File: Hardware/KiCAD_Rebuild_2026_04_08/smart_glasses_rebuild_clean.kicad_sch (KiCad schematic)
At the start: 12 parts

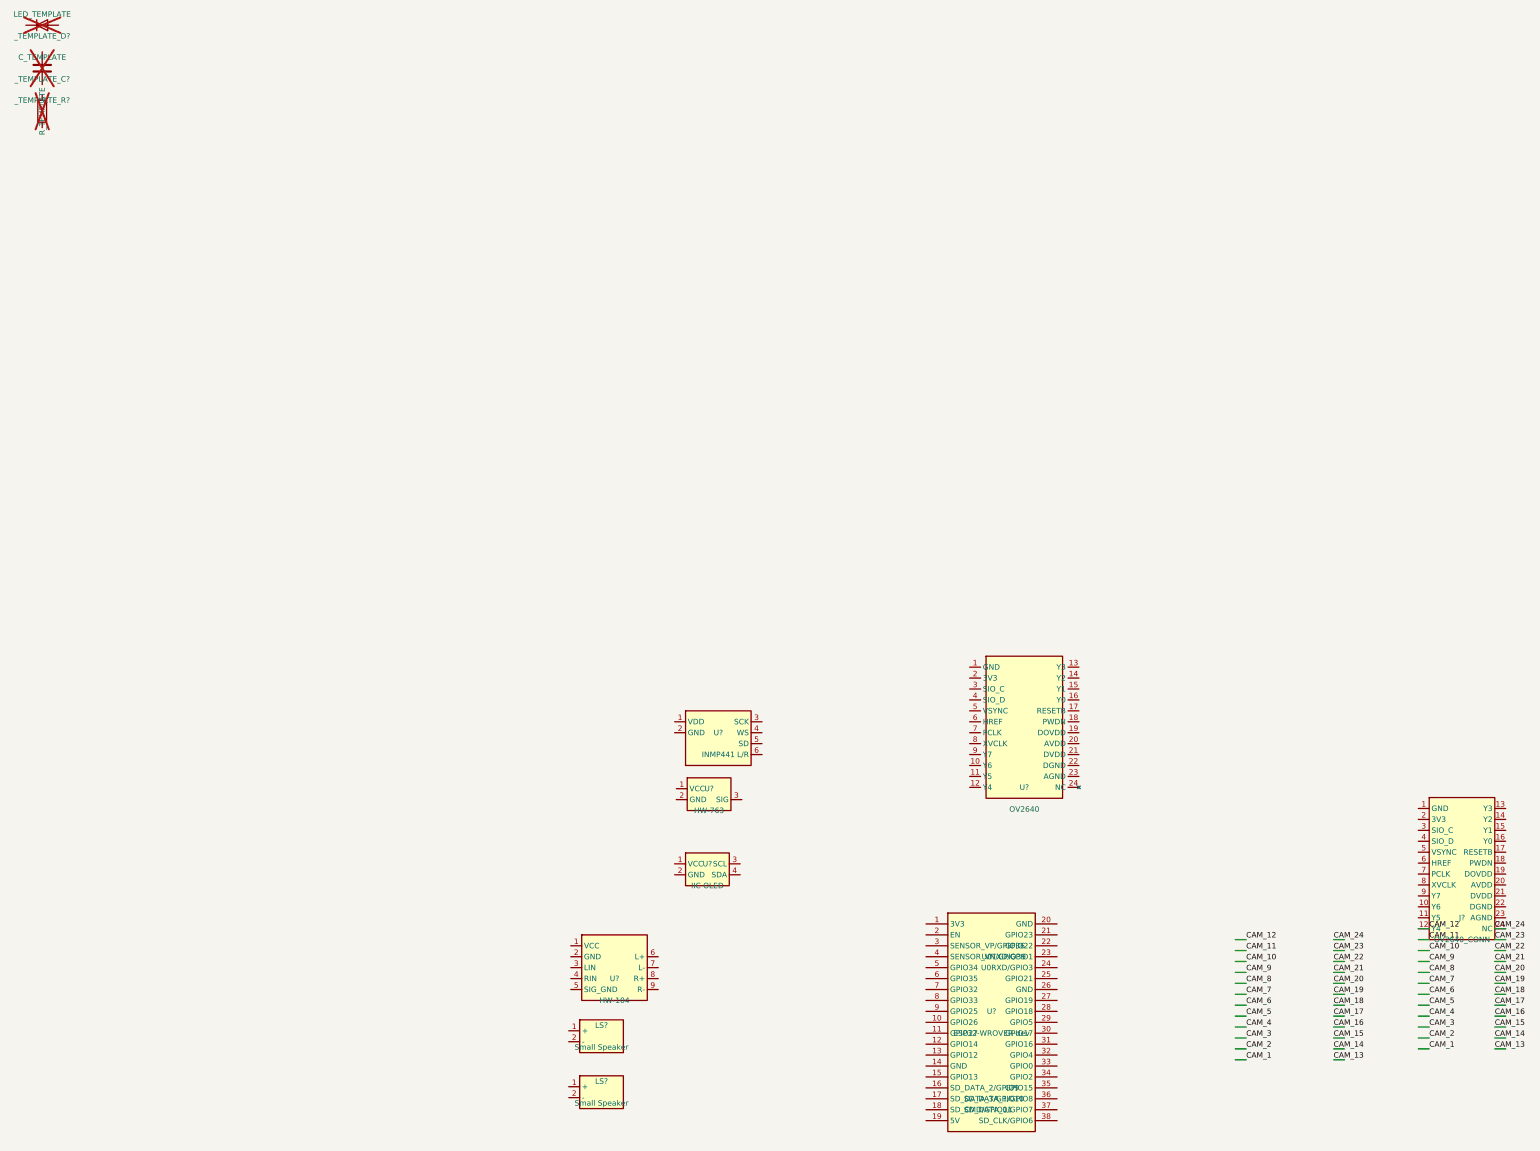
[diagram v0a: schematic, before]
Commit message: kicad manual checkpoint
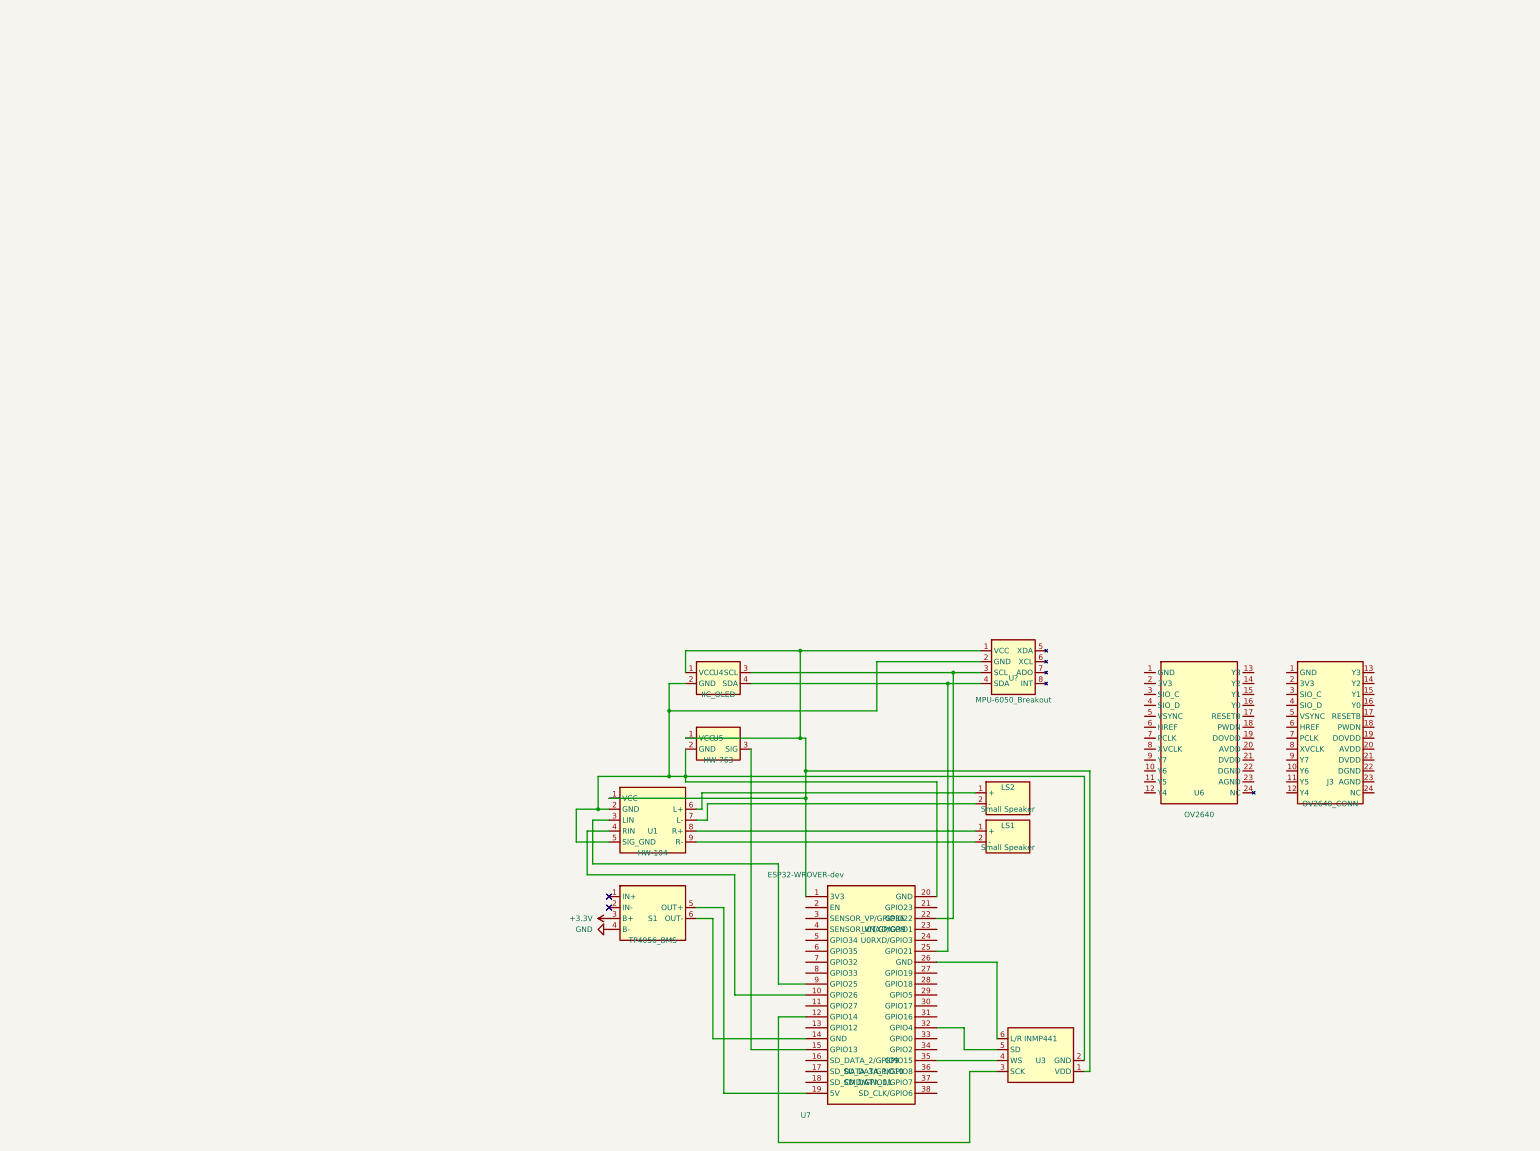
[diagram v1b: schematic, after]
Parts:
- removed J?: OV2640_CONN, symbol custom_symbols:OV2640_Connector_24Pin_Signal
- removed LS? (x2): Small Speaker, symbol custom_symbols:Speaker_Small_2Pin
- removed U?: OV2640, symbol custom_symbols:OV2640_Camera_Module_24P_Signal
- removed U?: HW-763, symbol custom_symbols:HW-763_Touch_Module
- removed U?: INMP441, symbol custom_symbols:INMP441_Mic_Module
- removed U?: ESP32-WROVER-dev, symbol custom_symbols:ESP32-WROVER-dev
- removed U?: IIC OLED, symbol custom_symbols:IIC_OLED_Module
- removed U?: HW-104, symbol custom_symbols:HW-104_Amplifier_Module_9P
- removed _TEMPLATE_C?: C_TEMPLATE, symbol Device:C
- removed _TEMPLATE_D?: LED_TEMPLATE, symbol Device:LED
- removed _TEMPLATE_R?: R_TEMPLATE, symbol Device:R
- added J3: OV2640_CONN, Connector_FFC-FPC:Hirose_FH12-24S-0.5SH_1x24-1MP_P0.50mm_Horizontal, symbol custom_symbols:OV2640_Connector_24Pin_Signal
- added LS1, LS2: Small Speaker, Connector_PinHeader_2.54mm:PinHeader_1x02_P2.54mm_Vertical, symbol custom_symbols:Speaker_Small_2Pin
- added S1: TP4056_BMS, Connector_PinHeader_2.54mm:PinHeader_1x06_P2.54mm_Vertical, symbol custom_symbols:TP4056_BMS_Module
- added U1: HW-104, Connector_PinHeader_2.54mm:PinHeader_1x09_P2.54mm_Vertical, symbol custom_symbols:HW-104_Amplifier_Module_9P
- added U3: INMP441, Connector_PinHeader_2.54mm:PinHeader_1x06_P2.54mm_Vertical, symbol custom_symbols:INMP441_Mic_Module
- added U4: IIC_OLED, Connector_PinHeader_2.54mm:PinHeader_1x04_P2.54mm_Vertical, symbol custom_symbols:IIC_OLED_Module
- added U5: HW-763, Connector_PinHeader_2.54mm:PinHeader_1x03_P2.54mm_Vertical, symbol custom_symbols:HW-763_Touch_Module
- added U6: OV2640, Connector_PinHeader_2.54mm:PinHeader_1x24_P2.54mm_Vertical, symbol custom_symbols:OV2640_Camera_Module_24P_Signal
- added U7: ESP32-WROVER-dev, Connector_PinHeader_2.54mm:PinHeader_2x19_P2.54mm_Vertical, symbol custom_symbols:ESP32-WROVER-dev
- added U?: MPU-6050_Breakout, Connector_PinHeader_2.54mm:PinHeader_1x08_P2.54mm_Vertical, symbol custom_symbols:MPU6050_Breakout_8P
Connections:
- new net: U1.1 (VCC), U3.1 (VDD), U4.1 (VCC), U5.1 (VCC), U7.1 (3V3), U?.1 (VCC)
- new net: U1.2 (GND), U1.5 (SIG_GND), U3.2 (GND), U4.2 (GND), U5.2 (GND), U7.20 (GND), U?.2 (GND)
- new net: U1.3 (LIN), U7.9 (GPIO25)
- new net: U1.4 (RIN), U7.10 (GPIO26)
- new net: LS2.1 (+), U1.6 (L+)
- new net: LS2.2 (-), U1.7 (L-)
- new net: LS1.1 (+), U1.8 (R+)
- new net: LS1.2 (-), U1.9 (R-)
- new net: U4.3 (SCL), U7.22 (GPIO22), U?.3 (SCL)
- new net: U4.4 (SDA), U7.25 (GPIO21), U?.4 (SDA)
- new net: U5.3 (SIG), U7.15 (GPIO13)
- new net: U3.3 (SCK), U7.12 (GPIO14)
- new net: S1.6 (OUT-), U7.14 (GND)
- new net: S1.5 (OUT+), U7.19 (5V)
- new net: U3.6 (L/R), U7.26 (GND)
- new net: U3.5 (SD), U7.32 (GPIO4)
- new net: U3.4 (WS), U7.35 (GPIO15)
- new net +3.3V: S1.3 (B+)
- new net GND: S1.4 (B-)
- no-connect marks 0 -> 2
